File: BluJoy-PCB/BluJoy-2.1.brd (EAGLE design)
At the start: 86.4 x 34.3 mm, 21 parts, among them J1 2468, Q1 P-FET, U1 PIC16F18446-I/SO, U2 HM-11, U3 3.0 LDO, U4 HM-11, X2 HB

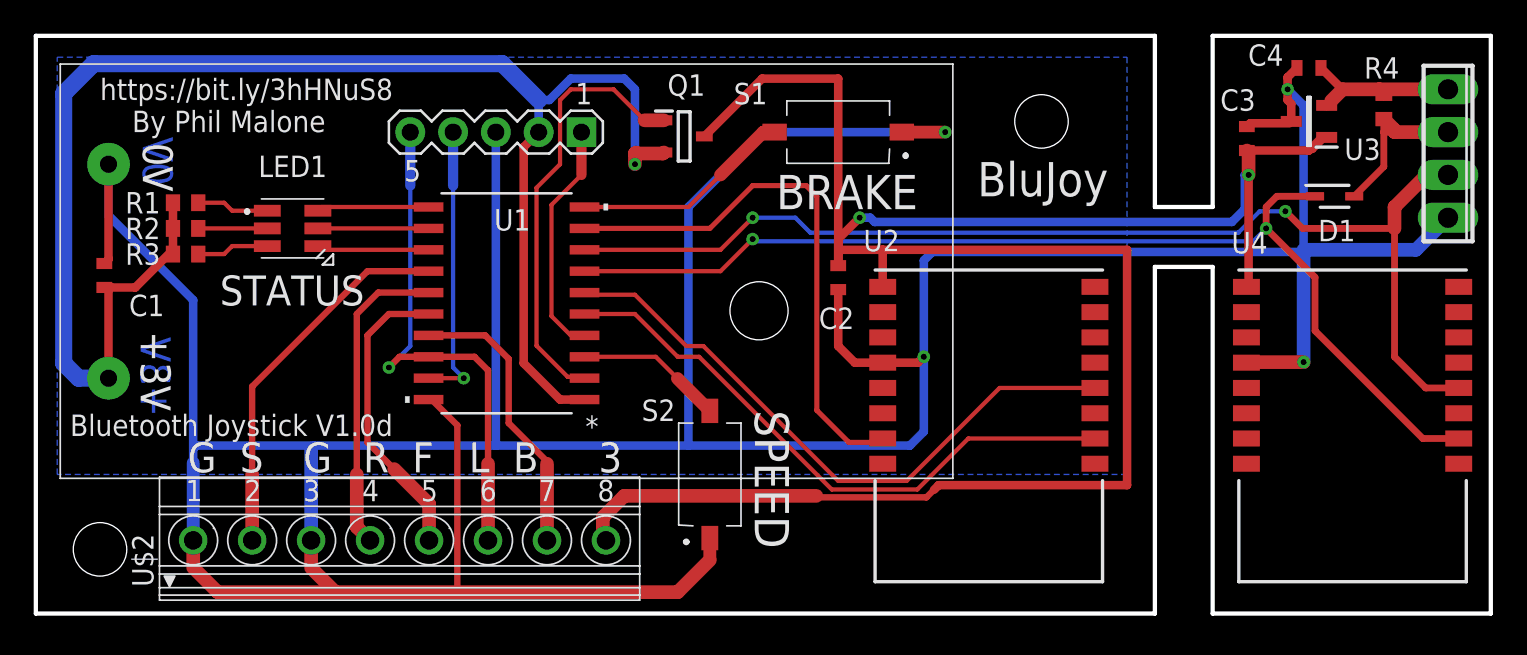
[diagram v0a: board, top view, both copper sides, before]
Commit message: Hackaday Prize Release.
Latest Firmware, Software, PCB and Cad.
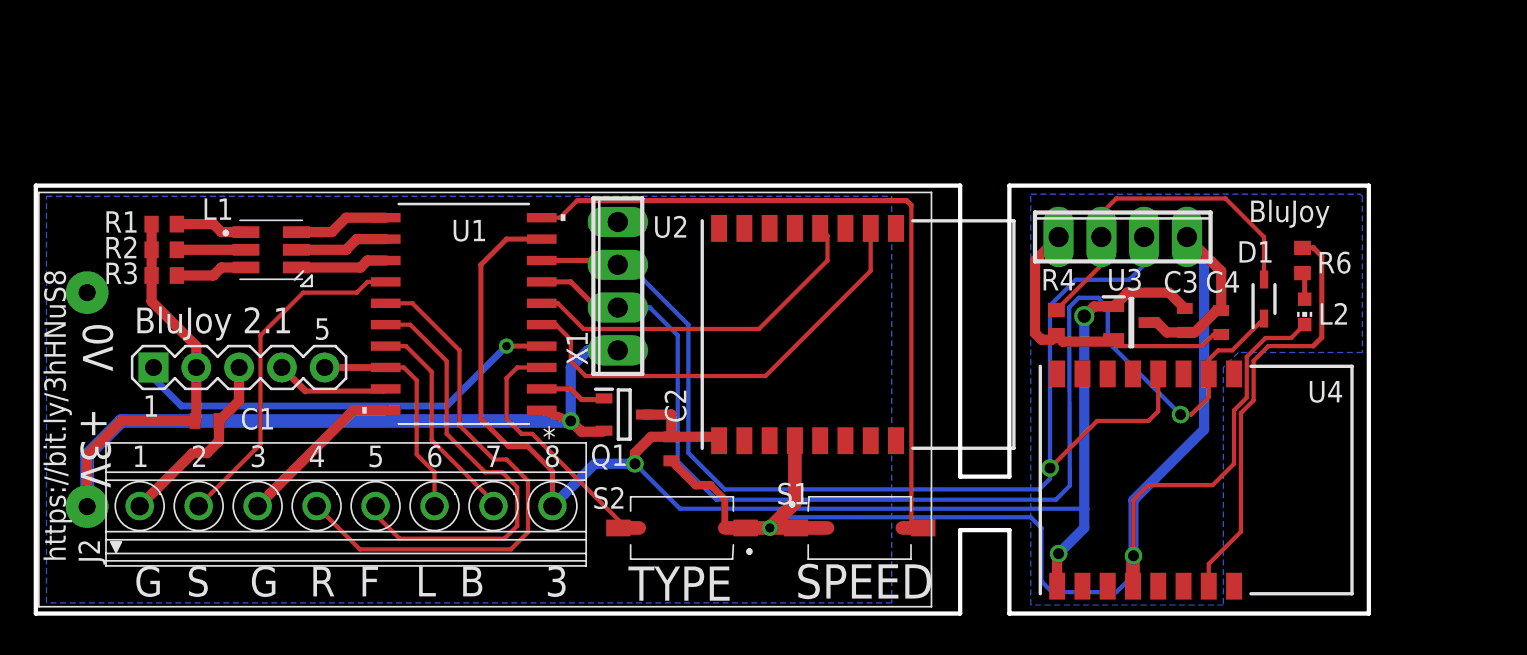
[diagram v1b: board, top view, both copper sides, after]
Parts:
- removed LED1: ASMB-TTF0-0A20B, BluJoy-e:ASMBTTF00A20B
- removed U$2: PHOENIX3.5X8-B, BluJoy-e:1751303
- added J2: PHOENIX3.5X8-B, BluJoy-e:1751303
- added L1: ASMB-TTF0-0A20B, BluJoy-e:ASMBTTF00A20B
- added L2: (no value), BluJoy-e:CHIP-LED0603
- added R6: 1K, BluJoy-e:RESC1608X50N
- added X1: HB, BluJoy-e:4POL254
- moved S1 23.5 mm to (48.9, 5.08), turned to 0 degrees
- moved R4 23.3 mm to (60.6, 17.3), turned to 90 degrees
- moved SV1 20.7 mm to (12.1, 14.6), turned to 0 degrees
- moved X2 19.9 mm to (64.5, 22.4), turned to 0 degrees
- moved U2 18.3 mm to (51.1, 22.9), turned to 270 degrees
- moved Q1 16.9 mm to (34.9, 11.8)
- moved C4 16.0 mm to (70.4, 17.3), turned to 270 degrees
- moved U3 15.9 mm to (65.0, 17.3), turned to 0 degrees
- moved U4 14.4 mm to (71.1, 14.2), turned to 270 degrees
- moved C2 14.2 mm to (37.7, 9.78)
- moved C3 11.4 mm to (68.2, 17.4), turned to 90 degrees
- moved C1 10.6 mm to (10.2, 11.4), turned to 180 degrees
- moved J1 7.73 mm to (26.7, 12.7)
- moved D1 7.40 mm to (72.9, 18.7), turned to 90 degrees
- moved S2 3.58 mm to (38.4, 5.08), turned to 180 degrees
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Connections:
- net POWER_ENA renamed !POWER_ENA1
- removed net CLK: SV1.5, U$2.6, U1.18
- removed net DOWN: U$2.7, U1.17
- removed net LED: U1.9, U2.15
- removed net RT/HOR: U$2.4, U1.15
- removed net UP/VERT: U$2.5, U1.16
- new net DOWN/VERT: J2.7, U1.17
- new net LEFT/HOR: J2.6, SV1.5, U1.18
- new net N$2: R6.2, U4.15
- new net N$3: L2.A, R6.1
- new net RT: J2.4, U1.15
- new net UP: J2.5, U1.16
- net 3V: now also X1.1
- net 3V-SW: now also J2.8, U1.9; no longer U$2.8
- net BLUE: now also L1.6; no longer LED1.6
- net ESTOP: now also J2.2; no longer U$2.2
- net GND: now also J2.1, J2.3, L2.C, X1.4; no longer U$2.1, U$2.3
- net GREEN: now also L1.4; no longer LED1.4
- net MASTER_RX: now also X1.3
- net MASTER_TX: now also X1.2
- net N$5: now also L1.1; no longer LED1.1
- net N$6: now also L1.3; no longer LED1.3
- net N$7: now also L1.5; no longer LED1.5
- net RED: now also L1.2; no longer LED1.2
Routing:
- net GND: track 281.2 -> 120.6 mm, vias 4 -> 2
- net 3V-SW: track 130.4 -> 87.4 mm, vias 2 -> 3
- net 3V: track 98.8 -> 66.2 mm
- net LED: track 32.6 -> 0.00 mm
- net RT: track 0.00 -> 32.5 mm
- net CLK: track 31.1 -> 0.00 mm, vias 1 -> 0
- net USER_1: track 13.1 -> 43.4 mm
- net UP: track 0.00 -> 26.4 mm
- net N$2: track 0.00 -> 25.3 mm
- net !POWER_ENA1: track 26.0 -> 3.99 mm
- net RT/HOR: track 18.5 -> 0.00 mm
- net UP/VERT: track 17.8 -> 0.00 mm
- net DOWN: track 17.0 -> 0.00 mm
- net SLAVE_RX: track 37.2 -> 21.4 mm
- net LEFT/HOR: track 0.00 -> 13.7 mm
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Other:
- board size 86.4 x 34.3 mm -> 79.1 x 25.4 mm
- board text added: "BluJoy 2.1"
- board text added: "TYPE"
- board text removed: "BRAKE"
- board text removed: "Bluetooth Joystick V1.0d"
- board text removed: "By Phil Malone"
- board text removed: "STATUS"
